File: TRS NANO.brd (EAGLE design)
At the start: 71.1 x 64.5 mm, 29 parts, among them M1 ARDUINO-NANO-3.0, Q5 BC548, Q6 BC548, Q7 BC548, Q8 BC548, T1 351, T2 LM35, T3 351, T41 351, T42 351

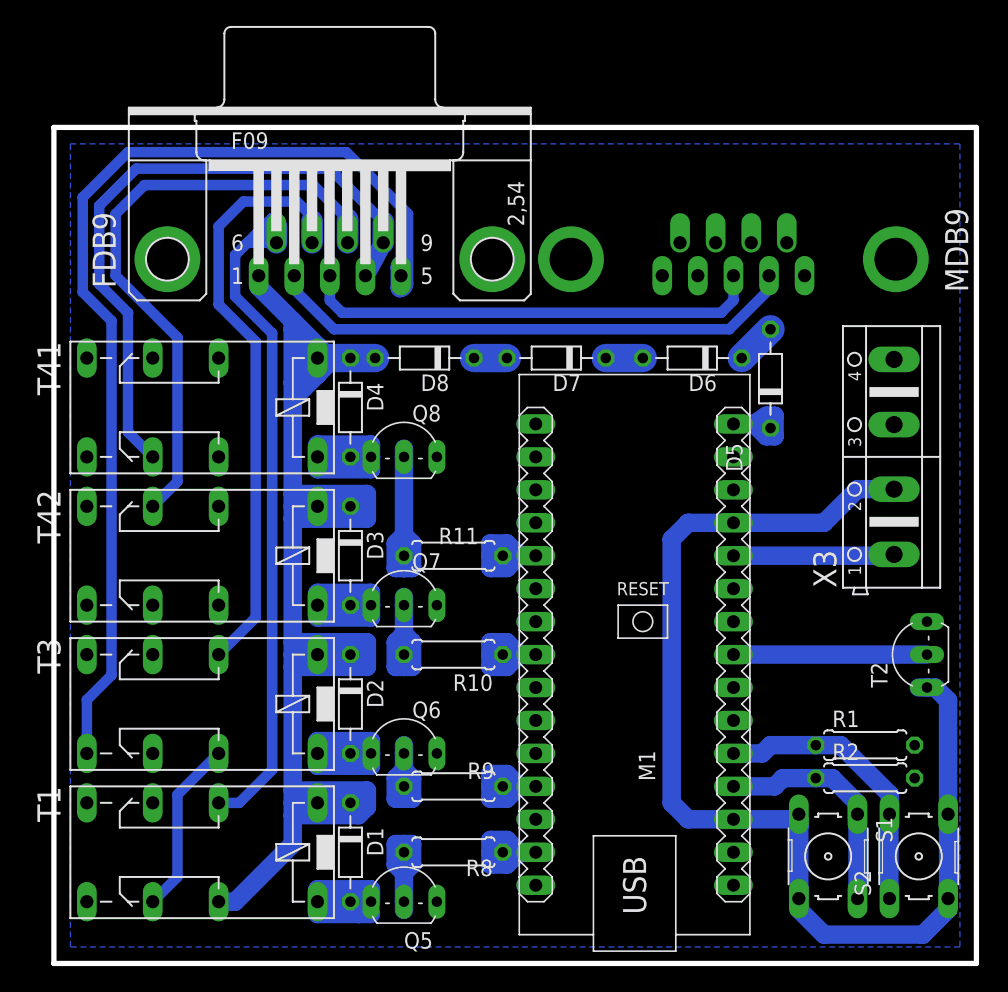
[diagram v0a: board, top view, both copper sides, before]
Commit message: PDFs
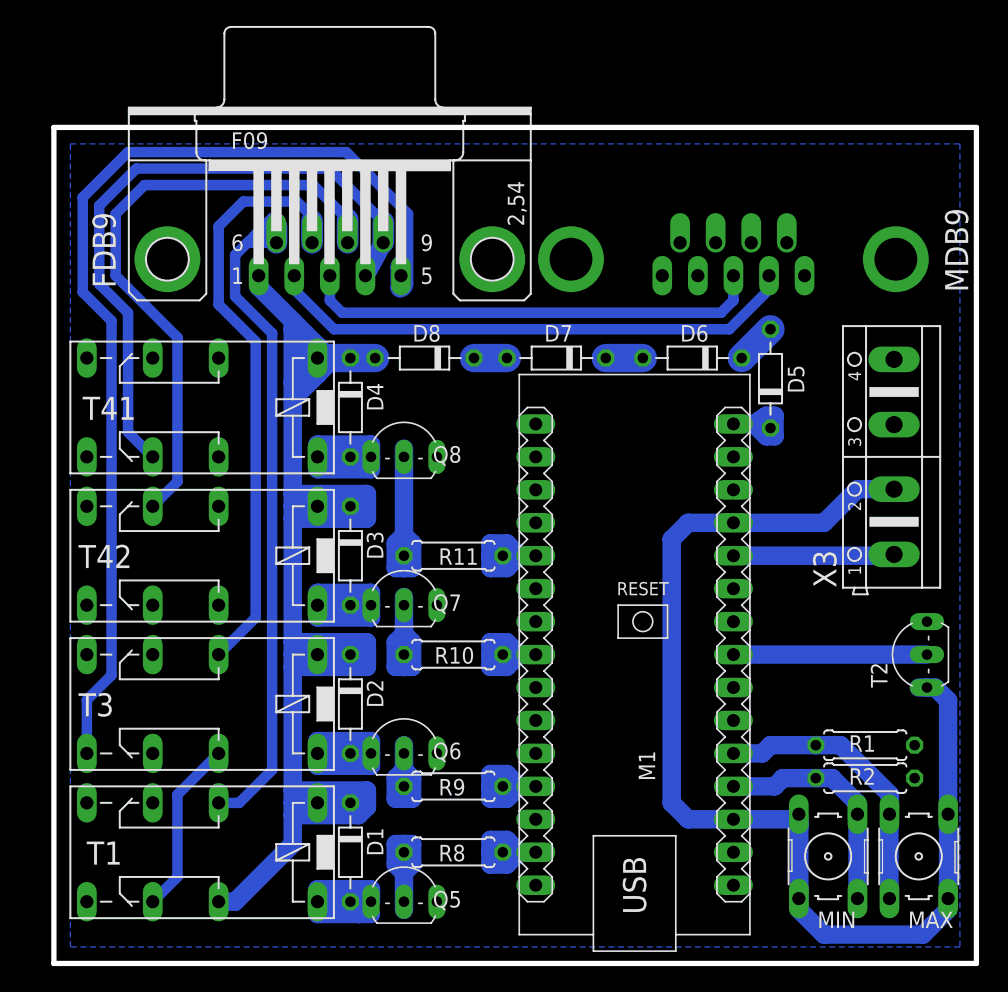
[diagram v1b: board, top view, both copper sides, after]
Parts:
- renumbered S1 to MIN, S2 to MAX
